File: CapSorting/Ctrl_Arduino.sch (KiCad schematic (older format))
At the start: 27 parts, among them J1 Conn_01x10, U1 TLP785, U13 TLP785, U2 TLP785

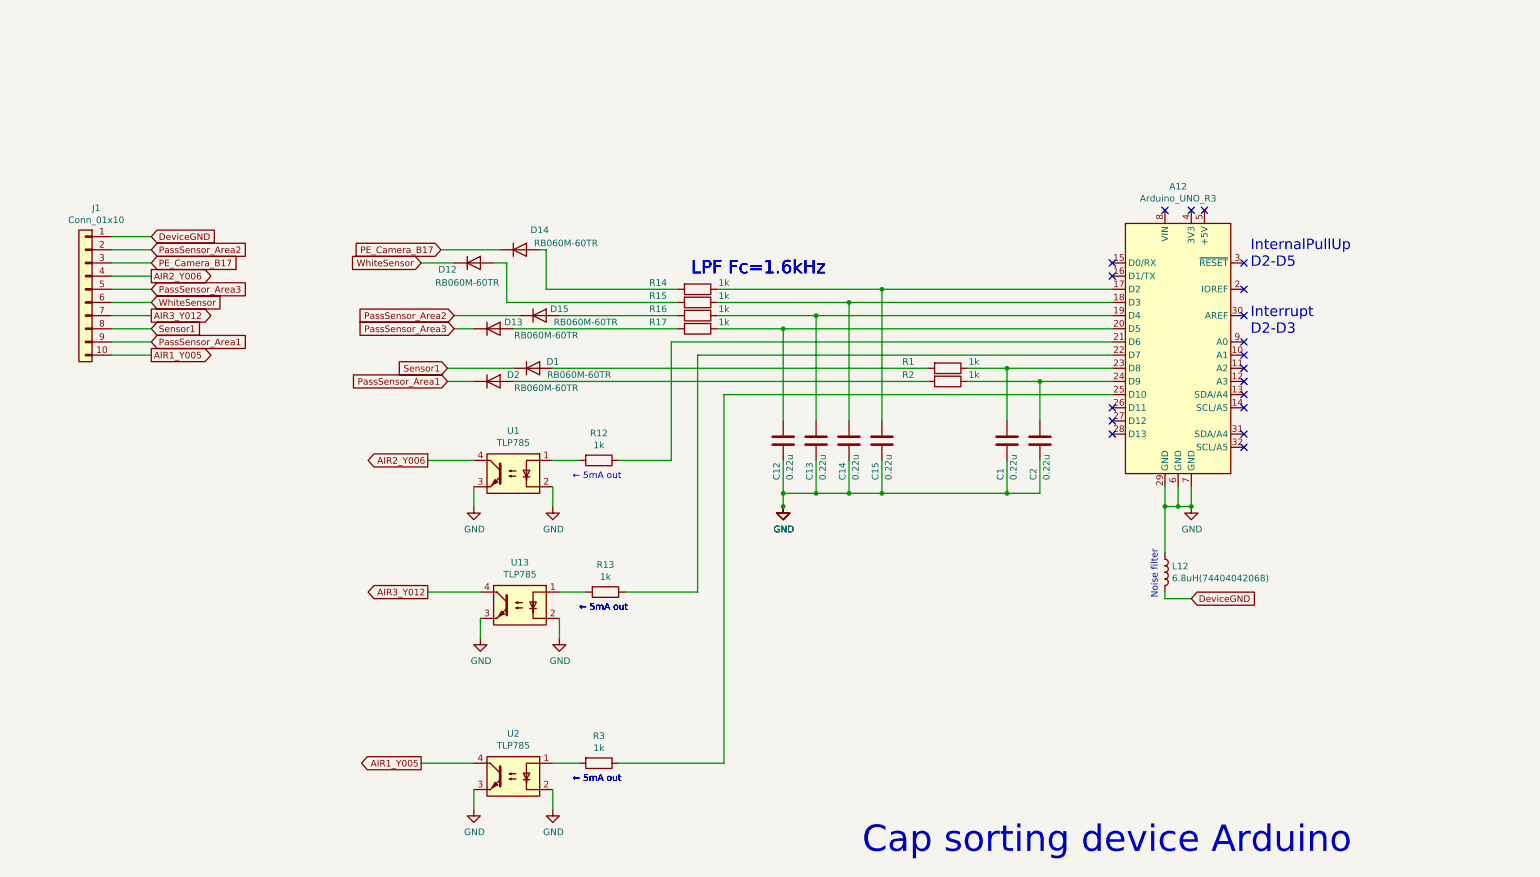
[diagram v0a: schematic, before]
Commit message: ガーバデータ追加
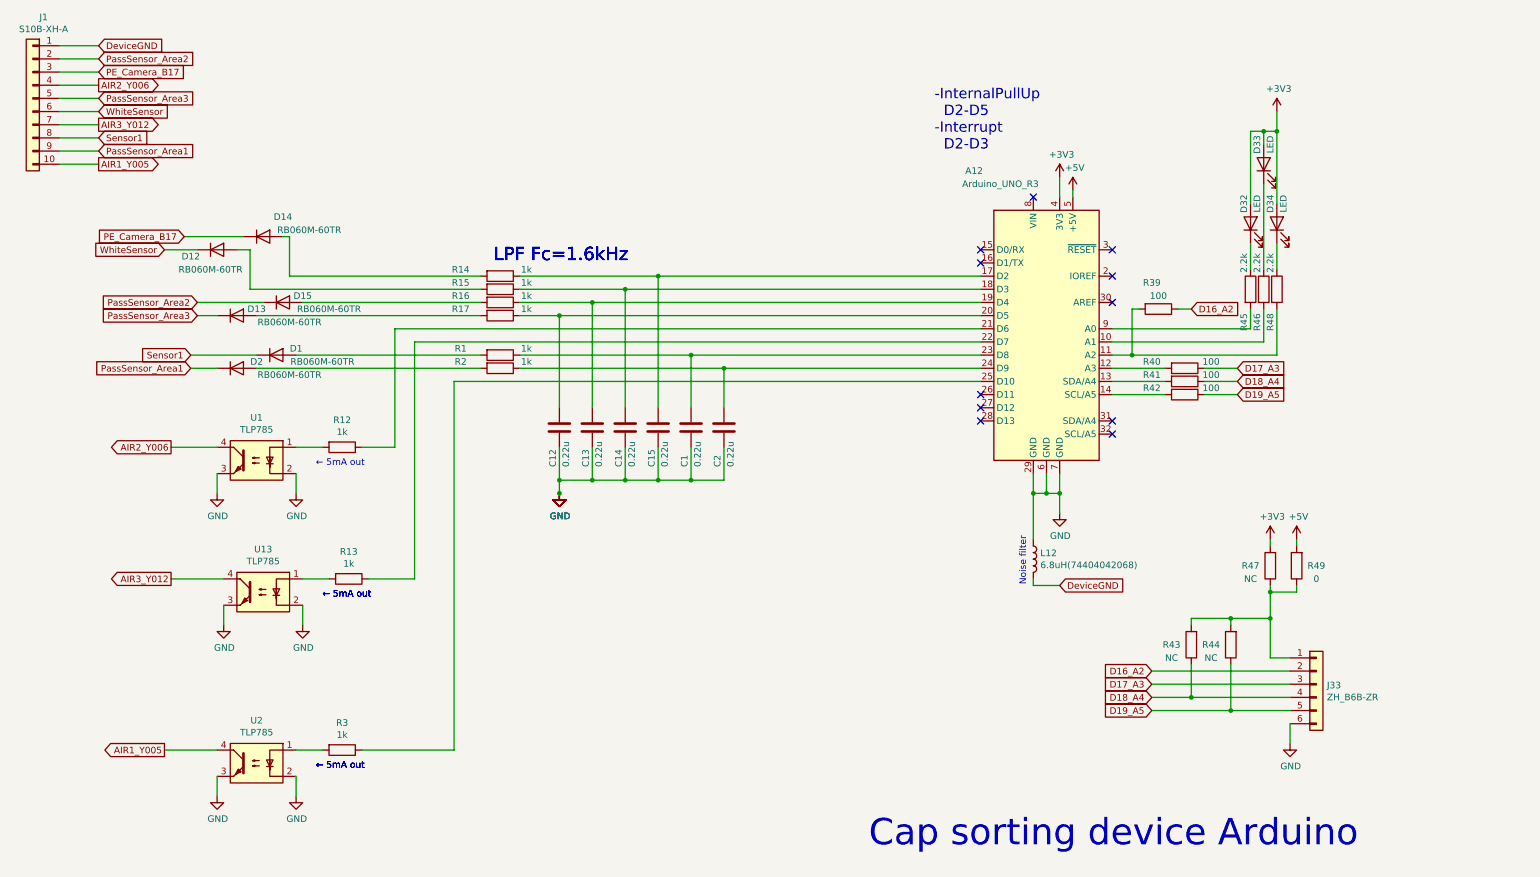
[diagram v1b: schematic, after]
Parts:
- added D32, D33, D34: LED, spot:LED1608, symbol Device:LED
- added J33: ZH_B6B-ZR, spot:ZH_B6B-ZR, symbol spot-cache:Connector_Generic_Conn_01x06
- added R39, R40, R41, R42: 100, Resistor_SMD:R_0603_1608Metric, symbol Device:R
- added R43, R44, R47: NC, Resistor_SMD:R_0603_1608Metric, symbol Device:R
- added R45, R46, R48: 2.2k, Resistor_SMD:R_0603_1608Metric, symbol Device:R
- added R49: 0, Resistor_SMD:R_0603_1608Metric, symbol Device:R
- J1: value Conn_01x10 -> S10B-XH-A; footprint JST:S10B-XH-A -> Connector_JST:JST_XH_S10B-XH-A_1x10_P2.50mm_Horizontal
- L12: footprint Ctrl_Arduino:INDPM4040X180N -> CapSorting:INDPM4040X180N
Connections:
- net GND: now also J33.6 (Pin_6)
- net at A12.10 (A1): now also R46.2
- net at A12.11 (A2): now also R39.2, R48.2
- net at A12.12 (A3): now also R40.2
- net at A12.13 (SDA/A4): now also R41.2
- net at A12.14 (SCL/A5): now also R42.2
- net +3V3: now reaches A12.4 (3V3)
- net +3V3: now also D32.2 (A), D33.2 (A), D34.2 (A), R47.2
- net +5V: now reaches A12.5 (+5V)
- net +5V: now also R49.2
- net at A12.9 (A0): now also R45.2
- new net: J33.1 (Pin_1), R43.2, R44.2, R47.1, R49.1
- new net: D32.1 (K), R45.1
- new net: D33.1 (K), R46.1
- new net: D34.1 (K), R48.1
- new net D16_A2: J33.2 (Pin_2), R39.1
- new net D17_A3: J33.3 (Pin_3), R40.1
- new net D18_A4: J33.4 (Pin_4), R41.1, R43.1
- new net D19_A5: J33.5 (Pin_5), R42.1, R44.1
- no-connect marks 19 -> 11
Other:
- note added: "-InternalPullUp\n D2-D5\n-Interrupt\n D2-D3"
- note removed: "InternalPullUp\nD2-D5\n\n\nInterrupt\nD2-D3"
- moved on the sheet: A12, C1, C12, C13, C14, C15, C2, D1, D12, D13, D14, D15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
